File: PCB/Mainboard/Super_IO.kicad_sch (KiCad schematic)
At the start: 24 parts, among them U22 FDC37C665IR, U23 EA, U25 E4

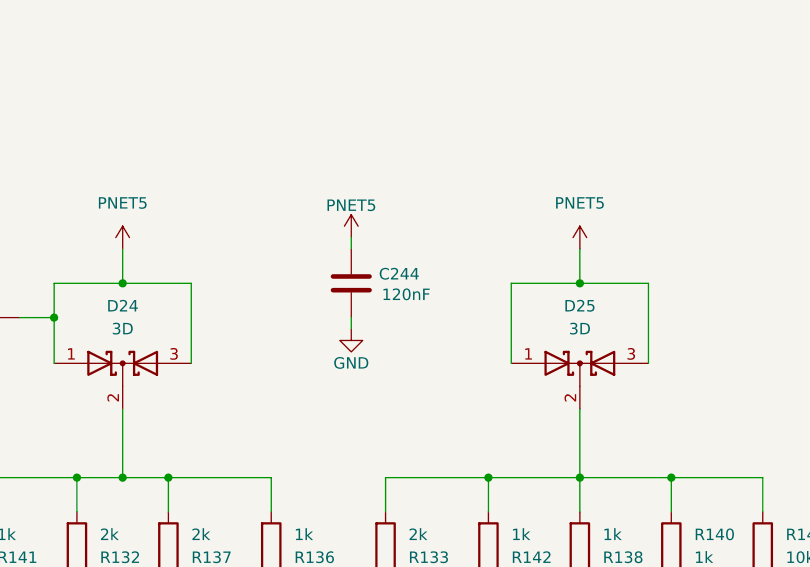
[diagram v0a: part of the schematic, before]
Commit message: Add files via upload
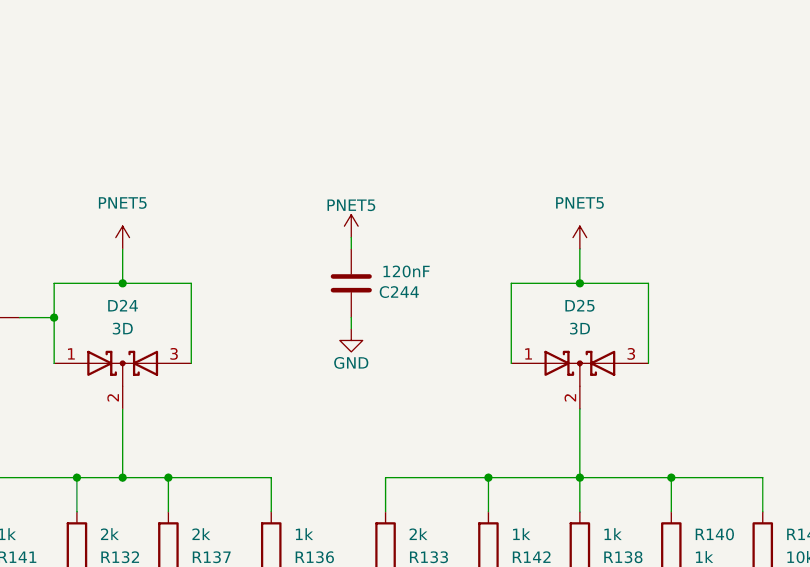
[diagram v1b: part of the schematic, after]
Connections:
- net GND: now also C244.1; no longer C244.2
- net PNET5: now also C244.2; no longer C244.1
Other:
- moved on the sheet: C244
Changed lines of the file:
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@@
 	(symbol
 		(lib_id "Device:C")
-		(at 312.42 81.28 0)
-		(mirror y)
+		(at 312.42 81.28 180)
 		(unit 1)
 		(exclude_from_sim no)
@@
 		(dnp no)
 		(property "Reference" "C244"
-			(at 317.754 80.264 0)
+			(at 317.754 82.296 0)
 			(effects
 				(font
@@
 		)
 		(property "Value" "120nF"
-			(at 318.516 82.55 0)
+			(at 318.516 80.01 0)
 			(effects
 				(font
@@
 		)
 		(property "Footprint" "Capacitor_SMD:C_0402_1005Metric"
-			(at 311.4548 85.09 0)
+			(at 311.4548 77.47 0)
 			(effects
 				(font
